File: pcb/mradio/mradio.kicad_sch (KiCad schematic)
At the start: 40 parts, among them U1 STM32H745ZITx

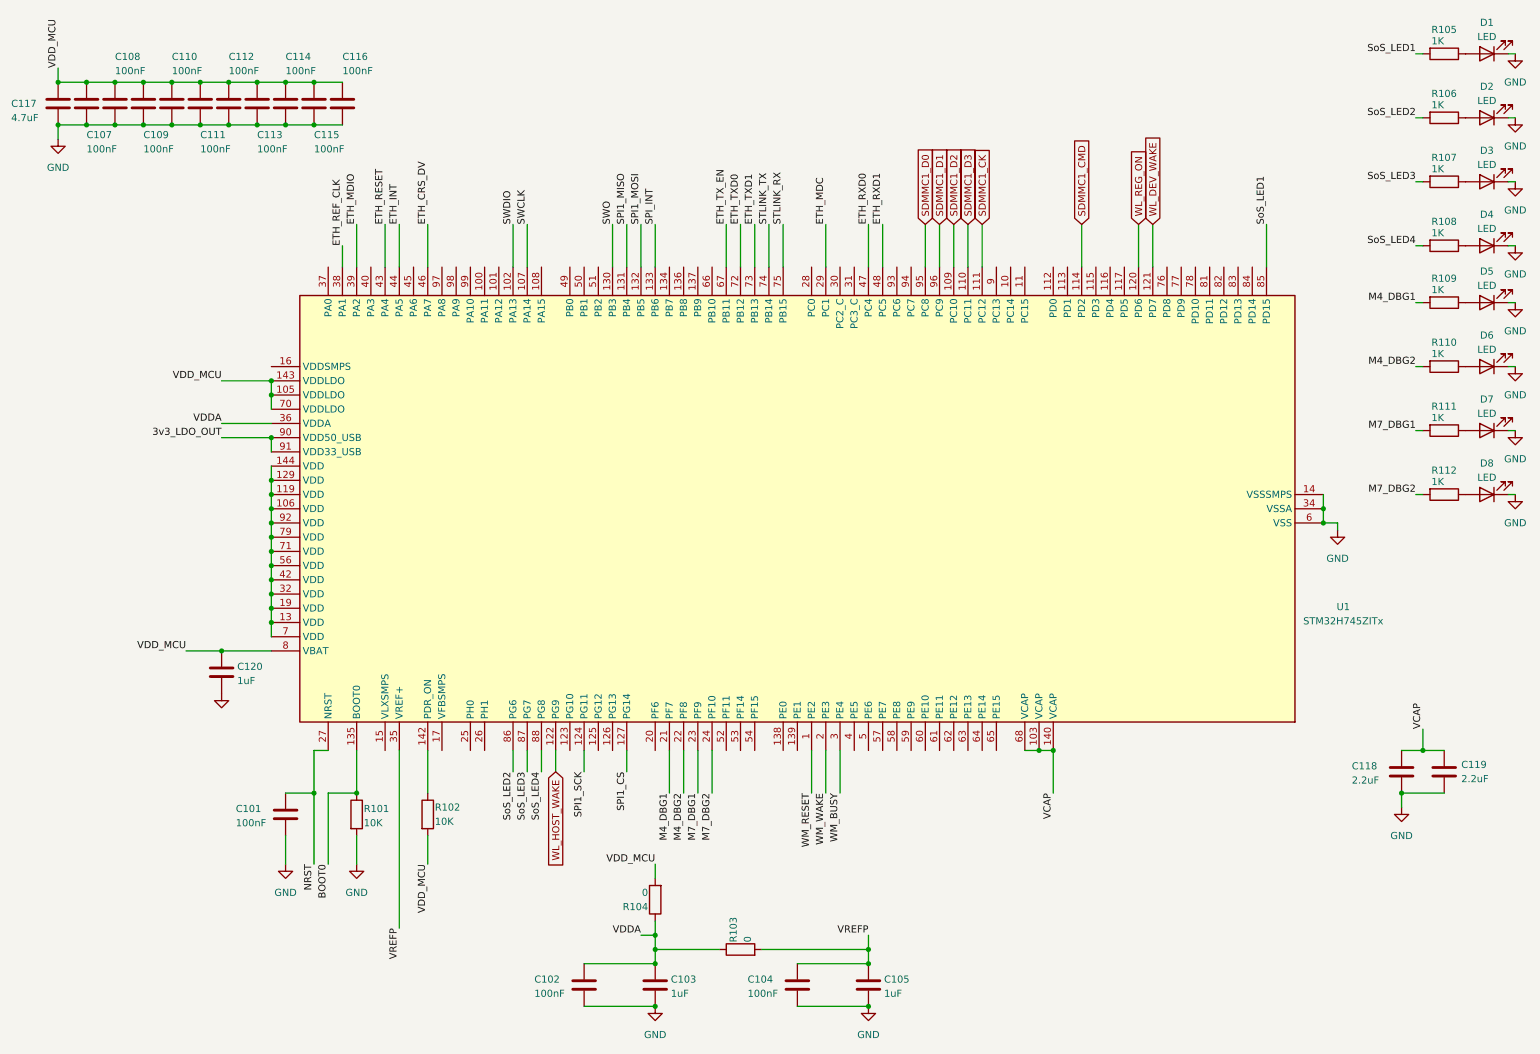
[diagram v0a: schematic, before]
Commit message: Fixed numbers
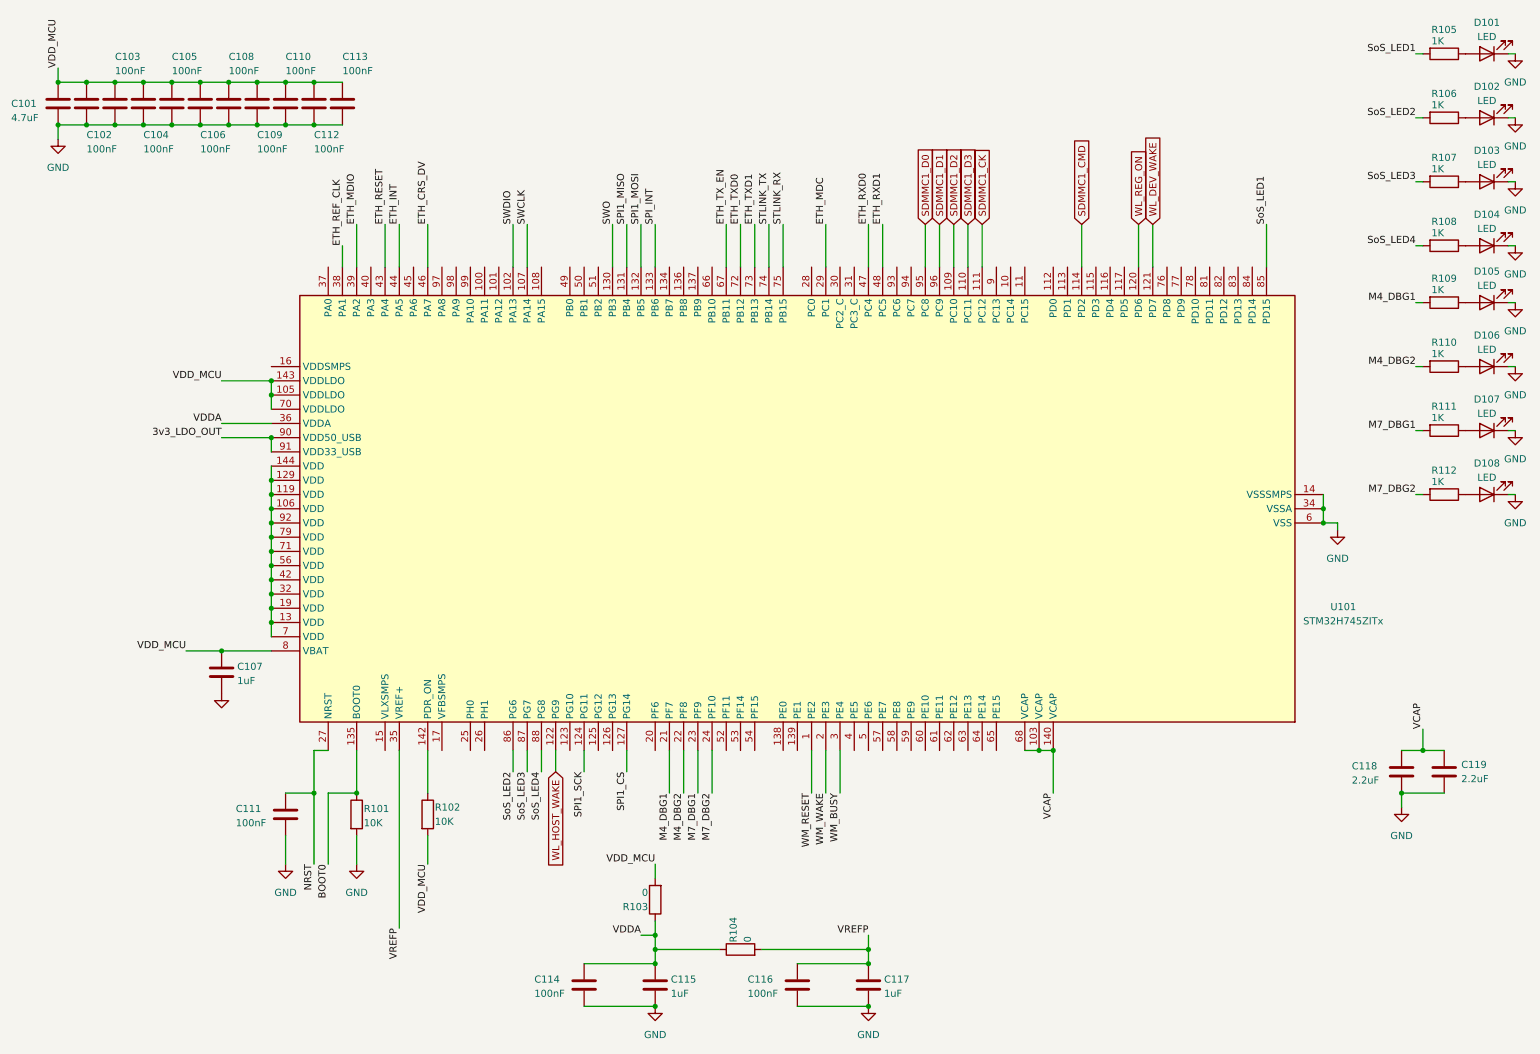
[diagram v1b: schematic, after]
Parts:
- renumbered C117 to C101, C107 to C102, C108 to C103, C109 to C104, C110 to C105, C111 to C106, C120 to C107, C112 to C108, C113 to C109, C114 to C110, C101 to C111, C115 to C112, C116 to C113, C102 to C114, C103 to C115, C104 to C116, C105 to C117, D1 to D101, D2 to D102, D3 to D103, D4 to D104, D5 to D105, D6 to D106, D7 to D107, D8 to D108, R104 to R103, R103 to R104, U1 to U101

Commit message: undid overwrite again
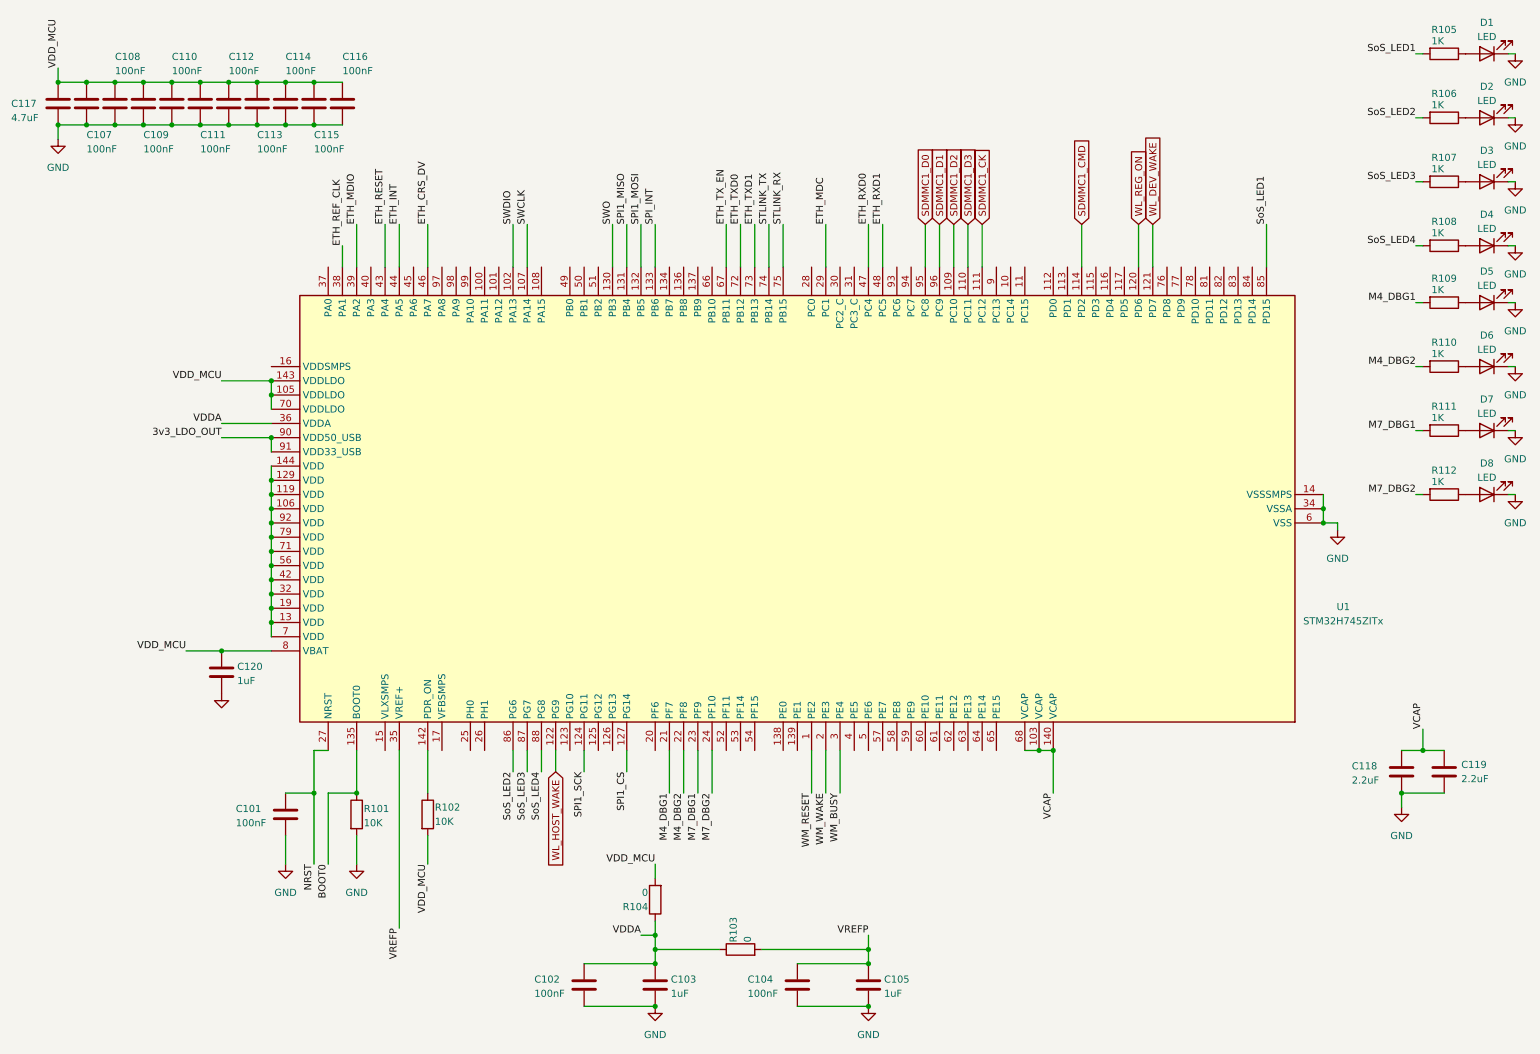
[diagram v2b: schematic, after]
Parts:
- renumbered C111 to C101, C114 to C102, C115 to C103, C116 to C104, C117 to C105, C102 to C107, C103 to C108, C104 to C109, C105 to C110, C106 to C111, C108 to C112, C109 to C113, C110 to C114, C112 to C115, C113 to C116, C101 to C117, C107 to C120, D101 to D1, D102 to D2, D103 to D3, D104 to D4, D105 to D5, D106 to D6, D107 to D7, D108 to D8, R104 to R103, R103 to R104, U101 to U1
